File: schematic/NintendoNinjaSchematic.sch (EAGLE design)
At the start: 6 parts, among them IC1 74165N, IC2 74LS04N

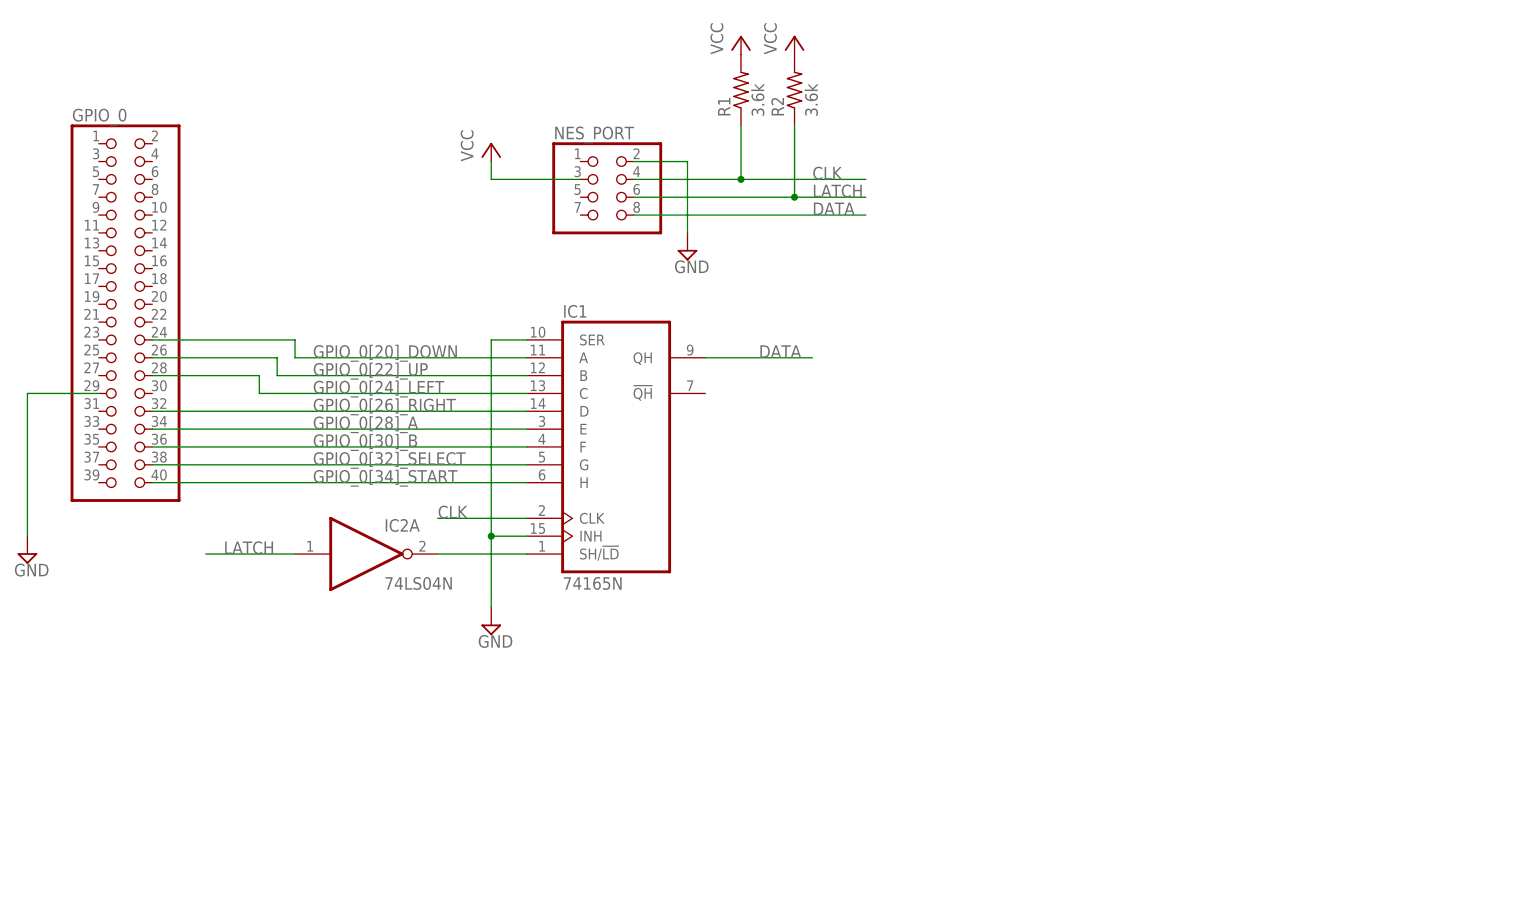
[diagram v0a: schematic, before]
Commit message: Further Content Updates, Schematic Completed.
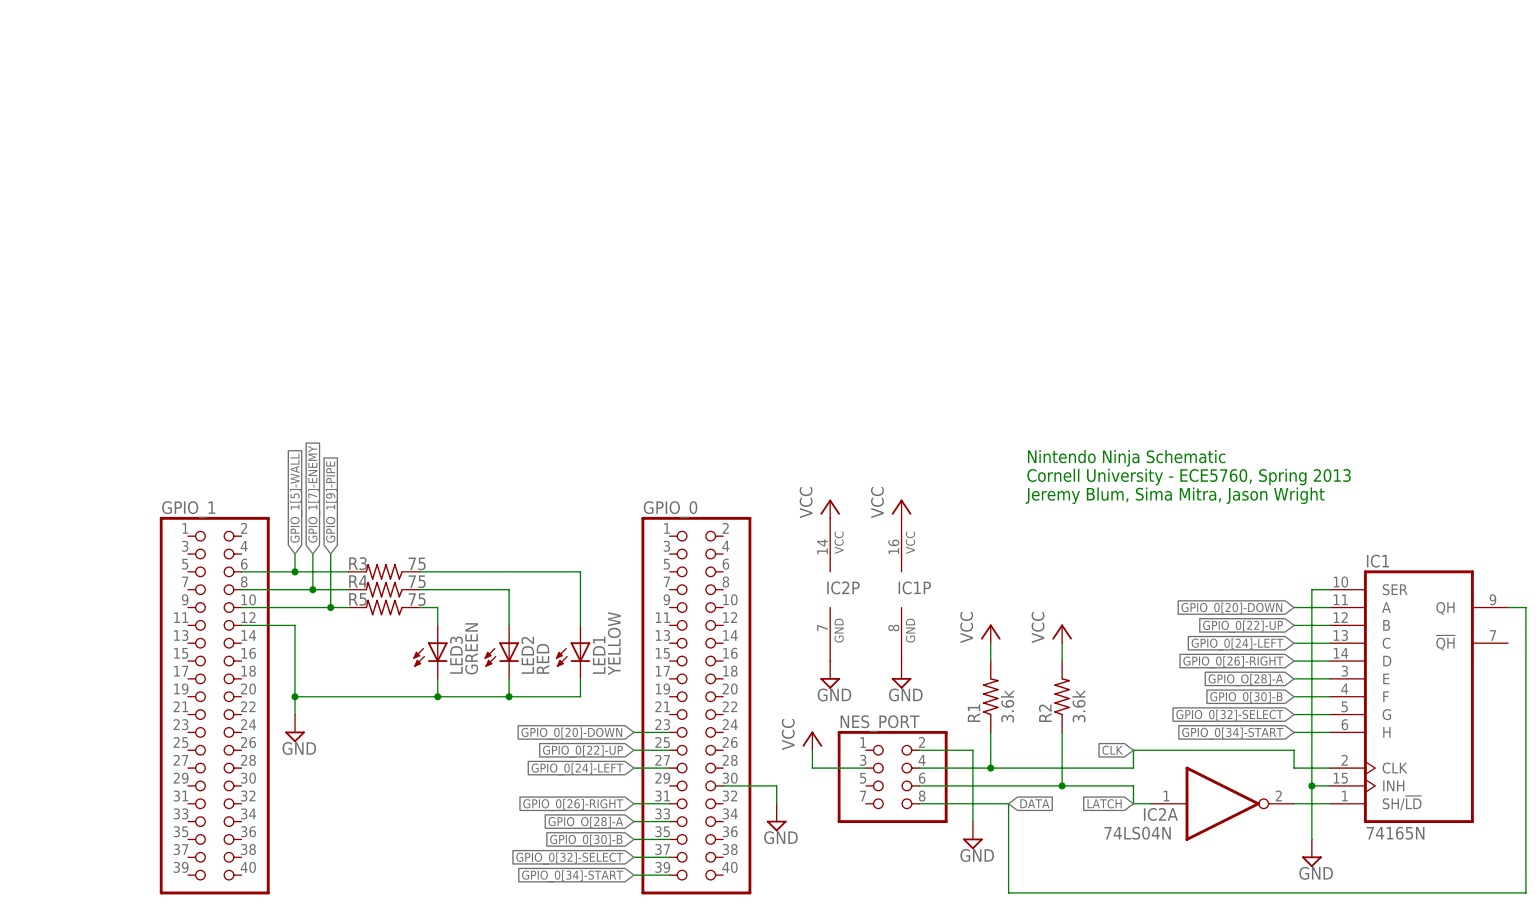
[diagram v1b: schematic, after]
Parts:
- added GPIO_1: (no value), pinhead:PINHD-2X20
- added LED1: YELLOW, adafruit:LED5MM
- added LED2: RED, adafruit:LED5MM
- added LED3: GREEN, adafruit:LED5MM
- added R3, R4, R5: 75, rcl:R-US_V526-0
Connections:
- removed net GPIO_0[20]_DOWN: GPIO_0.24, IC1A.A
- removed net GPIO_0[22]_UP: GPIO_0.26, IC1A.B
- removed net GPIO_0[24]_LEFT: GPIO_0.28, IC1A.C
- removed net GPIO_0[26]_RIGHT: GPIO_0.32, IC1A.D
- removed net GPIO_0[28]_A: GPIO_0.34, IC1A.E
- removed net GPIO_0[30]_B: GPIO_0.36, IC1A.F
- removed net GPIO_0[32]_SELECT: GPIO_0.38, IC1A.G
- removed net GPIO_0[34]_START: GPIO_0.40, IC1A.H
- new net GPIO_0[20]-DOWN: GPIO_0.23, IC1A.A
- new net GPIO_0[22]-UP: GPIO_0.25, IC1A.B
- new net GPIO_0[24]-LEFT: GPIO_0.27, IC1A.C
- new net GPIO_0[26]-RIGHT: GPIO_0.31, IC1A.D
- new net GPIO_0[30]-B: GPIO_0.35, IC1A.F
- new net GPIO_0[32]-SELECT: GPIO_0.37, IC1A.G
- new net GPIO_0[34]-START: GPIO_0.39, IC1A.H
- new net GPIO_1[5]-WALL: GPIO_1.6, R3.2
- new net GPIO_1[7]-ENEMY: GPIO_1.8, R4.2
- new net GPIO_1[9]-PIPE: GPIO_1.10, R5.2
- new net GPIO_O[28]-A: GPIO_0.33, IC1A.E
- new net N$1: LED3.A, R5.1
- new net N$2: LED2.A, R4.1
- new net N$3: LED1.A, R3.1
- net GND: now also GPIO_0.30, GPIO_1.12, IC1P.GND, IC2P.GND, LED1.C, LED2.C, LED3.C; no longer GPIO_0.29
- net VCC: now also IC1P.VCC, IC2P.VCC
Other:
- note added: "Nintendo Ninja Schematic Cornell University - ECE5760, Spring 2013 Jeremy Blum, Sima Mitra, Jason Wright"
- moved on the sheet: GPIO_0, IC1, IC2A, NES_PORT, R1, R2
